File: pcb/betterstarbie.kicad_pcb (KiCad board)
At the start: 2 copper layers, 80.5 x 95.9 mm, 7 parts, among them J1 Conn_01x04_Pin, J2 Conn_01x08_Pin, SW1 SW_Push, SW2 SW_Push, U1 DHT11, U2 XIAO-ESP32-C3-SMD

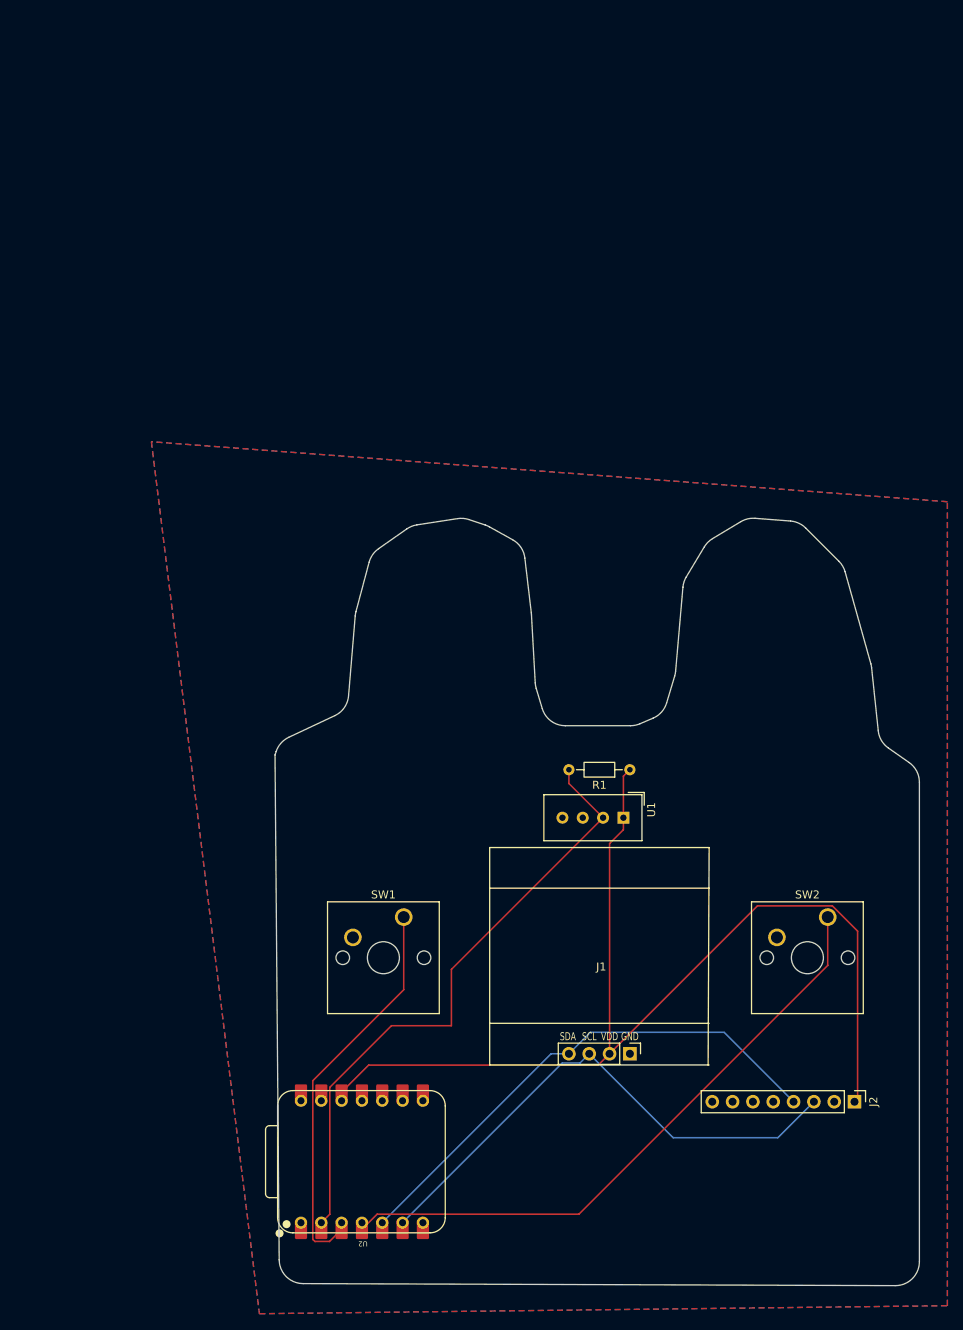
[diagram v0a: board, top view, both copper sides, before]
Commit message: Add files via upload
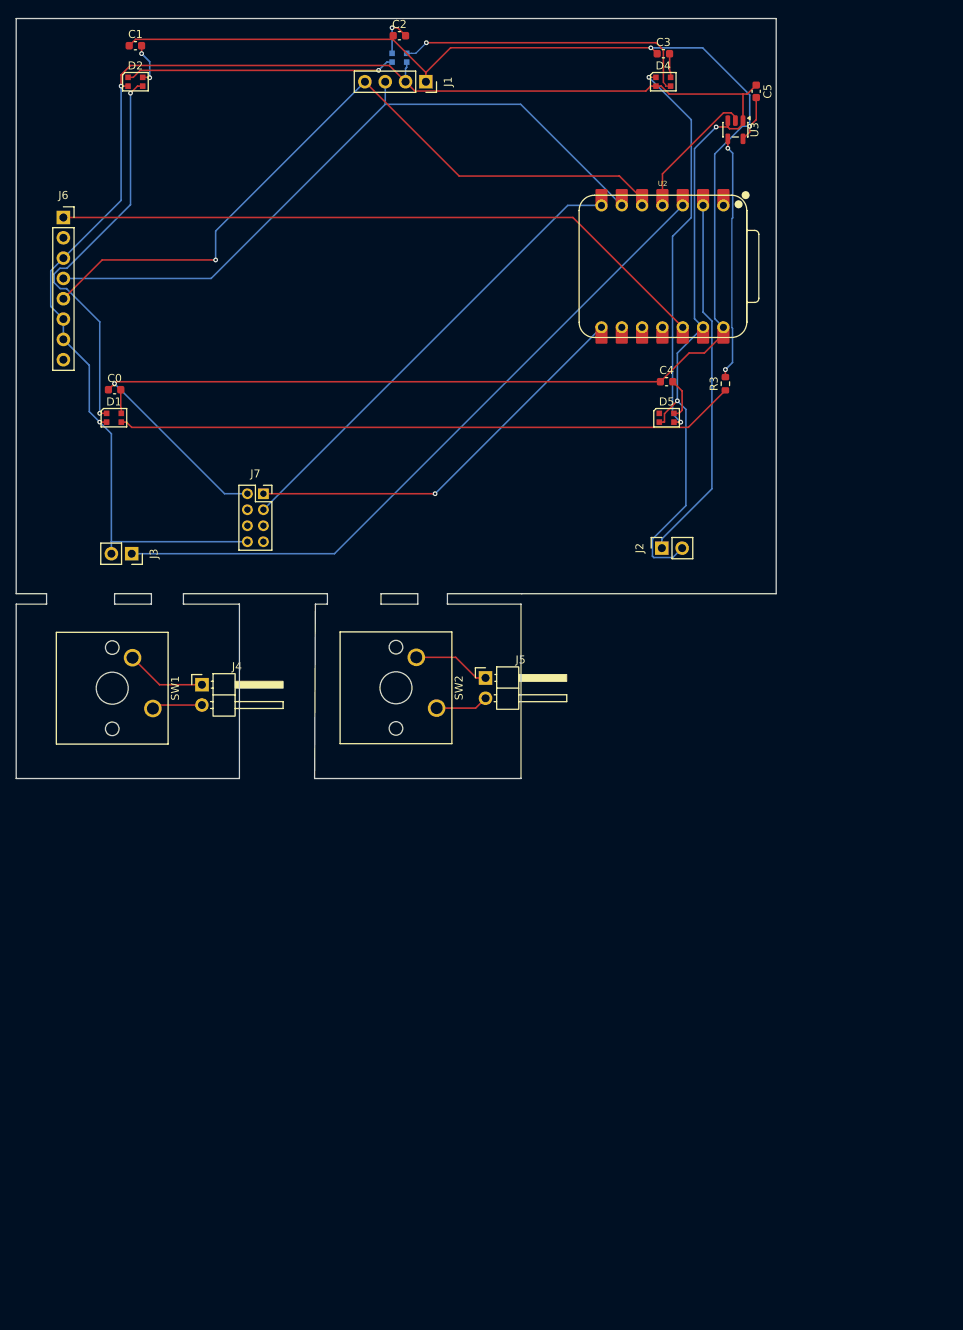
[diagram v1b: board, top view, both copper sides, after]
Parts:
- removed R1: 10k, Resistor_THT:R_Axial_DIN0204_L3.6mm_D1.6mm_P7.62mm_Horizontal
- removed U1: DHT11, Sensor:Aosong_DHT11_5.5x12.0_P2.54mm
- added C0: 100nF, Capacitor_SMD:C_0603_1608Metric, F.Cu at (24.4, 58.5)
- added C1: 100nF, Capacitor_SMD:C_0603_1608Metric, F.Cu at (27.0, 15.5)
- added C2: 100nF, Capacitor_SMD:C_0603_1608Metric, F.Cu at (60.0, 14.2)
- added C3: 100nF, Capacitor_SMD:C_0603_1608Metric, F.Cu at (93.0, 16.5)
- added C4: 100nF, Capacitor_SMD:C_0603_1608Metric, F.Cu at (93.4, 57.5)
- added C5: 100nF, Capacitor_SMD:C_0603_1608Metric, F.Cu at (104.6, 21.2)
- added D1: WS2812B-2020, LED_SMD:LED_WS2812B-2020_PLCC4_2.0x2.0mm, F.Cu at (24.3, 62.0)
- added D2: WS2812B-2020, LED_SMD:LED_WS2812B-2020_PLCC4_2.0x2.0mm, F.Cu at (27.0, 20.0)
- added D3: WS2812B-2020, LED_SMD:LED_WS2812B-2020_PLCC4_2.0x2.0mm, B.Cu at (60.0, 17.0)
- added D4: WS2812B-2020, LED_SMD:LED_WS2812B-2020_PLCC4_2.0x2.0mm, F.Cu at (93.0, 20.0)
- added D5: WS2812B-2020, LED_SMD:LED_WS2812B-2020_PLCC4_2.0x2.0mm, F.Cu at (93.4, 62.0)
- added J3: Conn_01x02_Socket, Connector_PinSocket_2.54mm:PinSocket_1x02_P2.54mm_Vertical, F.Cu at (26.5, 79.0)
- added J4: Conn_01x02_Pin, Connector_PinHeader_2.54mm:PinHeader_1x02_P2.54mm_Horizontal, F.Cu at (35.3, 95.4)
- added J5: Conn_01x02_Pin, Connector_PinHeader_2.54mm:PinHeader_1x02_P2.54mm_Horizontal, F.Cu at (70.8, 94.5)
- added J6: ENS160+AHT21, Connector_PinSocket_2.54mm:PinSocket_1x08_P2.54mm_Vertical, F.Cu at (18.0, 37.0)
- added J7: HLK-LD2450 2x4 2.00mm, Connector_PinSocket_2.00mm:PinSocket_2x04_P2.00mm_Vertical, F.Cu at (43.0, 71.5)
- added R3: 330Ω, Resistor_SMD:R_0603_1608Metric, F.Cu at (100.8, 57.8)
- added U3: 74AHCT1G125, Package_TO_SOT_SMD:SOT-23-5, F.Cu at (102.0, 26.0)
- J1: value Conn_01x04_Pin -> OLED_SH1107_1.5in; footprint Imported Parts:Display_128x64_096_I2C -> Connector_PinSocket_2.54mm:PinSocket_1x04_P2.54mm_Vertical
- J2: value Conn_01x08_Pin -> Conn_01x02_Socket; footprint Connector_PinHeader_2.54mm:PinHeader_1x08_P2.54mm_Vertical -> Connector_PinSocket_2.54mm:PinSocket_1x02_P2.54mm_Vertical
- U2: value XIAO-ESP32-C3-SMD -> XIAO-ESP32-S3-SMD; footprint Imported Parts:XIAO-ESP32-C6-DIP -> Seed Studio Library for Kicad:XIAO-ESP32-S3-DIP
- moved J1 123.4 mm to (63.3, 20.0), turned to -90 degrees
- moved U2 118.1 mm to (92.9, 43.1), turned to 0 degrees
- moved J2 73.3 mm to (92.8, 78.3), turned to 90 degrees
- moved SW2 55.4 mm to (64.7, 98.3), turned to -90 degrees
- moved SW1 40.8 mm to (29.2, 98.3), turned to -90 degrees
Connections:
- J1 pad 1: GND -> +5V
- J1 pad 2: +3.3V -> GND
- J2 pad 1: +3.3V -> /BTN1
- SW1 pad 1: /GPIO2 -> Net-(J4-Pin_2)
- SW1 pad 2: GND -> Net-(J4-Pin_1)
- SW2 pad 1: /GPIO3 -> Net-(J5-Pin_2)
- SW2 pad 2: GND -> Net-(J5-Pin_1)
- U2 pad 2: /DHT11 DATA -> /BTN1
- U2 pad 3: /GPIO2 -> /BTN2
- U2 pad 4: /GPIO3 -> /LED Data
- U2 pad 7: unconnected-(U2-D6-Pad7) -> /RADAR_TX
- U2 pad 8: unconnected-(U2-D7-Pad8) -> /RADAR_RX
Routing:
- net GND: track 0.83 -> 246.2 mm, vias 0 -> 4
- net +5V: track 0.00 -> 226.7 mm, vias 0 -> 3
- net /BTN2: track 0.00 -> 87.7 mm
- net /GPIO3: track 77.9 -> 0.00 mm
- net Net-(D1-DIN): track 0.00 -> 77.7 mm
- net /DHT11 DATA: track 77.4 -> 0.00 mm
- net /RADAR_TX: track 0.00 -> 58.9 mm
- net /RADAR_RX: track 0.00 -> 51.7 mm, vias 0 -> 1
- net +3.3V: track 134.6 -> 83.9 mm
- net Net-(D1-DOUT): track 0.00 -> 50.1 mm, vias 0 -> 2
- net /GPIO2: track 49.3 -> 0.00 mm
- net Net-(D4-DOUT): track 0.00 -> 48.4 mm, vias 0 -> 2
- net /BTN1: track 0.00 -> 46.7 mm
- net Net-(D3-DOUT): track 0.00 -> 38.3 mm, vias 0 -> 1
- net Net-(D2-DOUT): track 0.00 -> 33.8 mm, vias 0 -> 1
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- removed copper zone on B.Cu, net GND
- removed copper zone on F.Cu, net GND
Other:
- board size 80.5 x 95.9 mm -> 95 x 95 mm
- rule pad_to_mask_clearance: 0 -> 0.05
